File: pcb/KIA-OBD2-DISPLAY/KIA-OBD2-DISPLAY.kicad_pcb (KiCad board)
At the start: 4 copper layers, 132.1 x 19 mm, 58 parts, among them J1 Conn_01x07_Pin, J2 Conn_01x01, J3 Conn_01x01, J4 Conn_01x01, J5 Conn_01x01, J6 Conn_01x01, J7 Conn_01x01, J8 Conn_01x01, J9 Conn_01x01, P1 USB_C_Plug, Q1 BC817, U10 MCP2515-xST, U11 MCP2515-xST, U4 CAP1188-1-CP-TR, U6 TJA1050, U7 TJA1050, U9 ESP32-C6-MINI-1/U, Y1 Crystal_GND24_Small, Y4 Crystal_GND24_Small

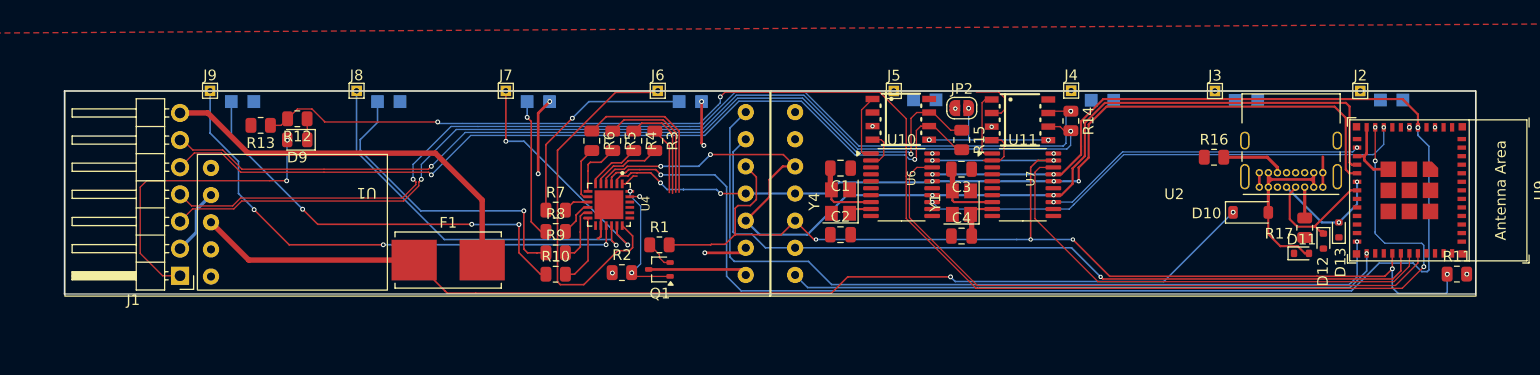
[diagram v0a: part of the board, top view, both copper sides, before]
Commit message: finall pcb
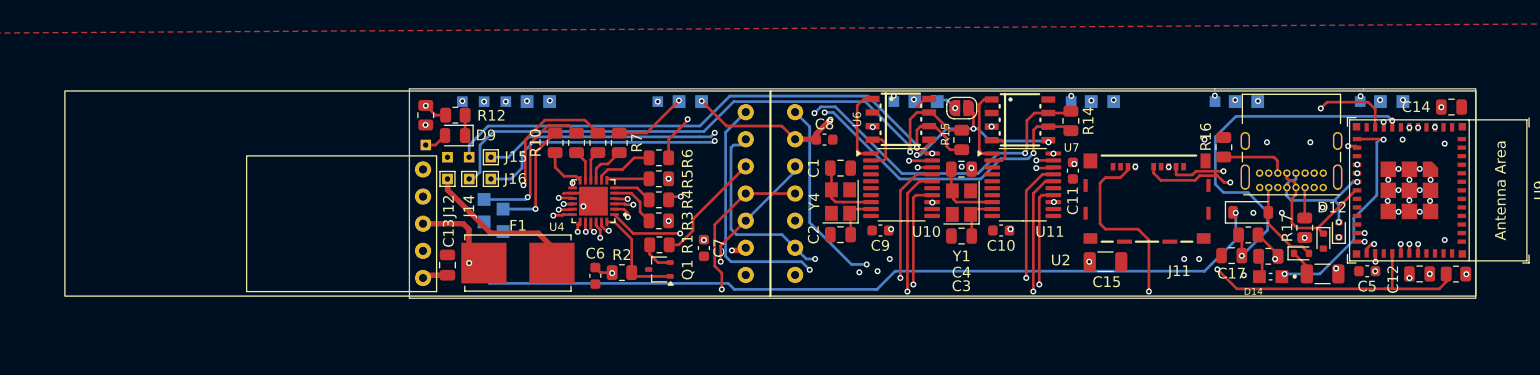
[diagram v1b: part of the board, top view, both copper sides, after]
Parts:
- removed J1: Conn_01x07_Pin, Connector_PinHeader_2.54mm:PinHeader_1x07_P2.54mm_Horizontal
- removed P1: USB_C_Plug, Connector_USB:USB_C_Receptacle_GCT_USB4085
- added C10: 100nF, Capacitor_SMD:C_0603_1608Metric, F.Cu at (181.0, 91.1)
- added C11: 100nF, Capacitor_SMD:C_0603_1608Metric, F.Cu at (187.7, 85.5)
- added C12: 10uF, Capacitor_SMD:C_0805_2012Metric, F.Cu at (220.2, 95.1)
- added C13: 10uF, Capacitor_SMD:C_0805_2012Metric, F.Cu at (129.2, 94.3)
- added C14: 10uF, Capacitor_SMD:C_0805_2012Metric, F.Cu at (223.1, 79.5)
- added C15: 100uF, Capacitor_SMD:C_1206_3216Metric, F.Cu at (190.8, 94.0)
- added C16: 100uF, Capacitor_SMD:C_1206_3216Metric, F.Cu at (211.1, 95.1)
- added C17: 10uF, Capacitor_SMD:C_0805_2012Metric, F.Cu at (202.6, 93.4)
- added C5: 100nF, Capacitor_SMD:C_0603_1608Metric, F.Cu at (215.3, 94.9)
- added C6: 100nF, Capacitor_SMD:C_0603_1608Metric, F.Cu at (143.0, 95.3)
- added C7: 100nF, Capacitor_SMD:C_0603_1608Metric, F.Cu at (153.2, 92.7)
- added C8: 100nF, Capacitor_SMD:C_0603_1608Metric, F.Cu at (164.5, 82.5)
- added C9: 100nF, Capacitor_SMD:C_0603_1608Metric, F.Cu at (169.7, 91.1)
- added D14: LED, LED_0602:LED_QBLP617-IW, F.Cu at (206.2, 95.4)
- added J10: USB_C_Receptacle_USB2.0_16P, Connector_USB:USB_C_Receptacle_GCT_USB4085, F.Cu at (211.1, 87.0)
- added J11: MEM2085-00-115-00-A_REV0.2, MEM2085:GCT_MEM2085-00-115-00-A_REV0.2, F.Cu at (194.6, 88.1)
- added J12: Conn_01x01, TestPoint:TestPoint_THTPad_1.0x1.0mm_Drill0.5mm, F.Cu at (129.2, 86.2)
- added J13: Conn_01x01, TestPoint:TestPoint_THTPad_1.0x1.0mm_Drill0.5mm, B.Cu at (131.2, 84.2)
- added J14: Conn_01x01, TestPoint:TestPoint_THTPad_1.0x1.0mm_Drill0.5mm, F.Cu at (131.2, 86.2)
- added J15: Conn_01x01, TestPoint:TestPoint_THTPad_1.0x1.0mm_Drill0.5mm, F.Cu at (133.2, 84.2)
- added J16: Conn_01x01, TestPoint:TestPoint_THTPad_1.0x1.0mm_Drill0.5mm, F.Cu at (133.2, 86.2)
- added J17: Conn_01x01, TestPoint:TestPoint_THTPad_1.0x1.0mm_Drill0.5mm, B.Cu at (129.2, 84.2)
- added J18: Conn_01x01, TestPoint:TestPoint_THTPad_1.0x1.0mm_Drill0.5mm, B.Cu at (127.1, 83.1)
- added R18: R, Resistor_SMD:R_0805_2012Metric, F.Cu at (206.0, 93.5)
- added R19: R, Resistor_SMD:R_0805_2012Metric, F.Cu at (204.1, 91.5)
- J2, J3, J4, J5, J6, J7, J8, J9: footprint TestPoint:TestPoint_THTPad_1.0x1.0mm_Drill0.5mm -> TestPoint:TestPoint_Pad_1.0x1.0mm; moved to B.Cu
- moved J2 43.7 mm to (170.9, 79.0), turned to 180 degrees
- moved J5 43.7 mm to (214.6, 79.0), turned to 180 degrees
- moved J9 41.9 mm to (148.8, 79.0), turned to 180 degrees
- moved D8 26.8 mm to (134.4, 90.1), turned to 90 degrees
- moved U8 25.8 mm to (128.1, 96.8), turned to 180 degrees
- moved J6 18.3 mm to (130.6, 79.0), turned to 180 degrees
- moved R13 15.5 mm to (127.1, 80.3), turned to -90 degrees
- moved R12 14.8 mm to (129.9, 80.3)
- moved D9 14.8 mm to (129.9, 82.2)
- moved J8 14.0 mm to (134.6, 79.0), turned to 180 degrees
- moved D7 13.6 mm to (132.6, 89.2), turned to 90 degrees
- moved J4 13.5 mm to (201.0, 79.0), turned to 180 degrees
- moved J3 13.5 mm to (187.5, 79.0), turned to 180 degrees
- moved R10 12.3 mm to (139.2, 82.9), turned to -90 degrees
- moved R9 10.5 mm to (141.2, 82.9), turned to -90 degrees
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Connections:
- U9 pad 12: unconnected-(U9-GPIO0/ADC1_CH0/XTAL_32K_P-Pad12) -> Net-(D14-A)
- U9 pad 23: unconnected-(U9-GPIO9-Pad23) -> /CSSDCARD
- U9 pad 30: /CSCAN2 -> /CSCAN
- U9 pad 31: /CSCAN -> /CSCAN2
- U9 pad 8: unconnected-(U9-EN/CHIP_PU-Pad8) -> Net-(U9-EN/CHIP_PU)
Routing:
- net /INTCAP: track 0.00 -> 87.6 mm, vias 1 -> 2
- net Net-(J5-Pin_1): track 0.00 -> 87.3 mm, vias 0 -> 2
- net /CSCAP: track 1.68 -> 77.0 mm, vias 0 -> 2
- net Net-(D1-K): track 6.31 -> 78.3 mm, vias 0 -> 2
- net Net-(J4-Pin_1): track 0.00 -> 68.5 mm, vias 0 -> 2
- net Net-(J3-Pin_1): track 0.00 -> 56.7 mm, vias 0 -> 2
- net /MOSI: track 82.9 -> 138.1 mm, vias 5 -> 6
- net Net-(D2-K): track 9.92 -> 59.1 mm, vias 0 -> 2
- net /INTING: track 141.7 -> 94.8 mm, vias 5 -> 2
- net Net-(J2-Pin_1): track 0.00 -> 37.7 mm, vias 0 -> 2
- net Net-(U9-EN/CHIP_PU): track 0.00 -> 35.8 mm, vias 0 -> 2
- net /MISO: track 154.3 -> 119.5 mm, vias 4 -> 5
- net /CAN LISTEN H: track 97.2 -> 62.9 mm, vias 2 -> 3
- net Net-(J9-Pin_1): track 48.8 -> 15.8 mm, vias 3 -> 2
- net Net-(D3-K): track 12.4 -> 42.6 mm, vias 0 -> 2
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- added copper zone on In2.Cu, net +3.3V
- added copper zone on In1.Cu, net GND
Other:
- board size 132.1 x 19 mm -> 99.8 x 19.6 mm
- rule pad_to_mask_clearance: 0 -> 0.038
- rule solder_mask_min_width: 0.1016 -> 0.1

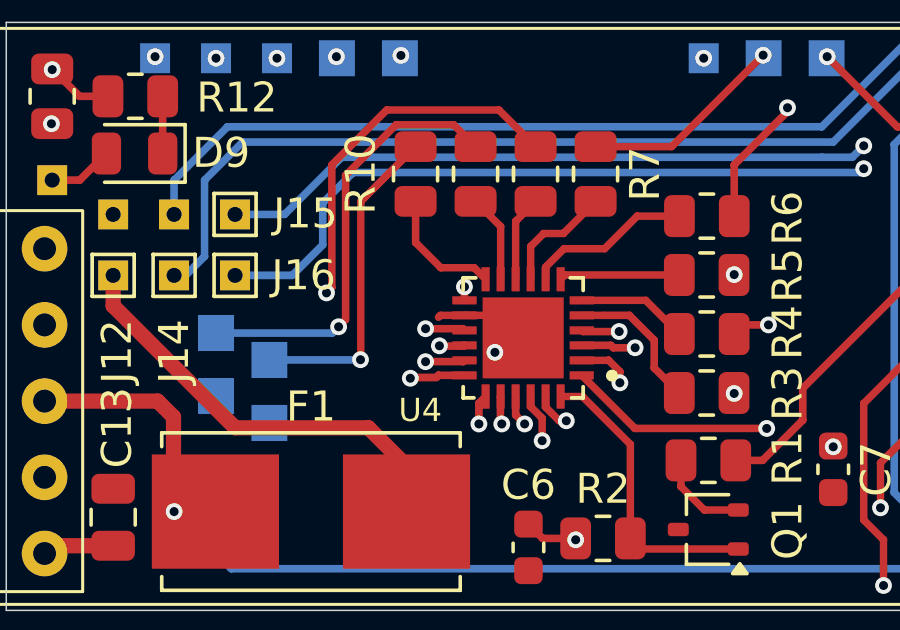
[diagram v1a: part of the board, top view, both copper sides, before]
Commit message: deps and pcb update
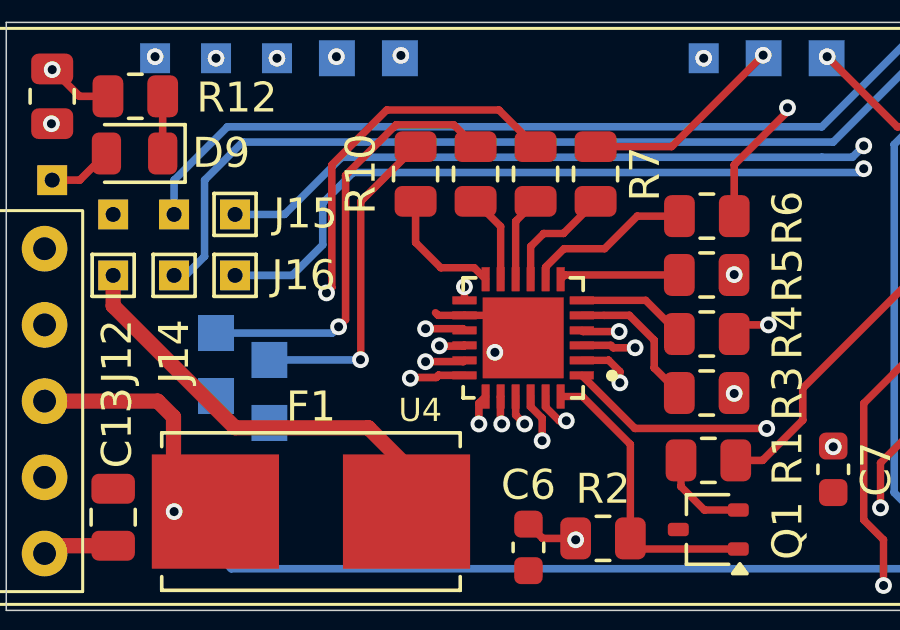
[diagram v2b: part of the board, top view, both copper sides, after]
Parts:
- R10, R18, R3, R4, R5, R6, R7, R8, R9: value R -> 65R
- R11, R19: value R -> 10k
- R12: value R -> 4.7k
- R13: value R -> 1k
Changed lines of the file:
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@@
 			(layer "F.SilkS")
 		)
-		(fp_text user "${REFERENCE}"
-			(at 9.948955 6.206265 180)
-			(unlocked yes)
-			(layer "F.Fab")
-			(effects
-				(font
-					(size 1 1)
-					(thickness 0.15)
-				)
-			)
-		)
 		(pad "1" thru_hole circle
 			(at 1.27 1.27 180)
@@
 			)
 		)
-		(property "Value" "R"
+		(property "Value" "65R"
 			(at 0 1.65 0)
 			(layer "F.Fab")
@@
 			(at 0 4.2 0)
 			(layer "F.Fab")
+			(hide yes)
 			(effects
 				(font
@@
 			)
 		)
-		(property "Value" "R"
+		(property "Value" "65R"
 			(at 0 1.65 90)
 			(layer "F.Fab")
+			(hide yes)
 			(effects
 				(font
@@
 			(at 0 2.45 -90)
 			(layer "F.Fab")
+			(hide yes)
 			(effects
 				(font
@@
 			(at 0 4.2 0)
 			(layer "F.Fab")
+			(hide yes)
 			(effects
 				(font
@@
 		)
 		(property "Value" "22pF"
-			(at 0 1.68 180)
+			(at 2.754282 0.12994 -90)
 			(layer "F.Fab")
 			(effects
@@
 			)
 		)
-		(property "Value" "R"
+		(property "Value" "65R"
 			(at 0 1.65 0)
 			(layer "F.Fab")
+			(hide yes)
 			(effects
 				(font
@@
 		)
 		(property "Value" "100nF"
-			(at 0 1.43 0)
+			(at -0.902 -1.778 0)
 			(layer "F.Fab")
 			(effects
@@
 			)
 		)
-		(property "Value" "R"
+		(property "Value" "65R"
 			(at 0 1.65 0)
 			(layer "F.Fab")
+			(hide yes)
 			(effects
 				(font
@@
 			)
 		)
-		(property "Value" "R"
+		(property "Value" "65R"
 			(at 0 1.65 90)
 			(layer "F.Fab")
@@
 		)
 		(property "Value" "TJA1050"
-			(at 6.5 0.5 90)
+			(at -4.119 -0.003 180)
 			(layer "F.Fab")
 			(effects
@@
 		)
 		(property "Value" "100nF"
-			(at 0 1.43 0)
+			(at -0.114 -1.778 0)
 			(layer "F.Fab")
 			(effects
@@
 			(at 7.95 1.95 180)
 			(layer "F.Fab")
+			(hide yes)
 			(effects
 				(font
@@
 		)
 		(property "Value" "5.1k"
-			(at 0 1.65 90)
+			(at -1.858128 1.804804 90)
 			(layer "F.Fab")
 			(effects
@@
 			(at 0 1.85 0)
 			(layer "F.Fab")
-			(hide yes)
 			(effects
 				(font
@@
 			)
 		)
-		(property "Value" "R"
+		(property "Value" "10k"
 			(at 0 1.65 0)
 			(layer "F.Fab")
@@
 		)
 		(property "Value" "SD05_SOD323"
-			(at 0 1.4 0)
+			(at -3.995 5.86 0)
 			(layer "F.Fab")
-			(hide yes)
 			(effects
 				(font
@@
 		)
 		(fp_text user "${REFERENCE}"
-			(at 0 -1.3 0)
+			(at -1.963 -1.633 0)
 			(layer "F.Fab")
 			(effects
@@
 		)
 		(property "Value" "100nF"
-			(at 0 1.43 90)
+			(at 3.823 0 90)
 			(layer "F.Fab")
 			(effects
@@
 		)
 		(property "Value" "100nF"
-			(at 0 1.43 0)
+			(at -1.257 -1.778 0)
 			(layer "F.Fab")
 			(effects
@@
 			)
 		)
-		(property "Value" "R"
-			(at 0 1.65 0)
+		(property "Value" "65R"
+			(at 0 3.81 0)
 			(layer "F.Fab")
 			(effects
@@
 			)
 		)
-		(property "Value" "R"
+		(property "Value" "65R"
 			(at 0 1.65 0)
 			(layer "F.Fab")
+			(hide yes)
 			(effects
 				(font
@@
 		)
 		(property "Value" "10uF"
-			(at 0 1.68 0)
+			(at 1.649364 -2.224239 0)
 			(layer "F.Fab")
 			(effects
@@
 		)
 		(property "Value" "100nF"
-			(at 0 1.43 0)
+			(at -0.876 -1.778 0)
 			(layer "F.Fab")
 			(effects
@@
 		)
 		(property "Value" "22pF"
-			(at 0 1.68 180)
+			(at -0.018646 -1.678598 0)
 			(layer "F.Fab")
 			(effects
@@
 		)
 		(property "Value" "TJA1050"
-			(at 6.5 0.5 90)
+			(at -4.069 0.020975 180)
 			(layer "F.Fab")
 			(effects
@@
 		)
 		(property "Value" "100uF"
-			(at 0 1.85 0)
+			(at 0 -2.032 0)
 			(layer "F.Fab")
 			(effects
@@
 		)
 		(fp_text user "${REFERENCE}"
-			(at 0 -1.3 -90)
+			(at 0.068 2.665 0)
 			(layer "F.Fab")
 			(effects
@@
 		)
 		(property "Value" "5.1k"
-			(at 0 1.65 -90)
+			(at 1.646 -1.755 -90)
 			(layer "F.Fab")
-			(hide yes)
 			(effects
 				(font
@@
 		)
 		(property "Value" "10uF"
-			(at 0 1.68 0)
+			(at -0.315 -2.159 0)
 			(layer "F.Fab")
 			(effects
@@
 		)
 		(fp_text user "${REFERENCE}"
-			(at 0 -1.3 90)
+			(at -2.769 0.076 -90)
 			(layer "F.Fab")
 			(effects
@@
 		)
 		(property "Value" "10uF"
-			(at 0 1.68 0)
+			(at 0 -1.905 0)
 			(layer "F.Fab")
 			(effects
@@
 		)
 		(property "Value" "BC817"
-			(at -0.05 2.05 180)
+			(at -0.227313 -2.57776 180)
 			(layer "F.Fab")
 			(effects
@@
 			)
 		)
-		(property "Value" "R"
+		(property "Value" "4.7k"
 			(at 0 1.65 180)
 			(layer "F.Fab")
@@
 			)
 		)
-		(property "Value" "R"
+		(property "Value" "1k"
 			(at 0 1.65 90)
 			(layer "F.Fab")
@@
 		)
 		(property "Value" "120R"
-			(at 0 1.65 90)
+			(at 0.224859 -1.972484 90)
 			(layer "F.Fab")
 			(effects
@@
 			(at 12.85 -5.315 0)
 			(layer "F.Fab")
+			(hide yes)
 			(effects
 				(font
@@
 			)
 		)
-		(property "Value" "R"
+		(property "Value" "65R"
 			(at 0 1.65 90)
 			(layer "F.Fab")
+			(hide yes)
 			(effects
 				(font
@@
 			(at 0 2.45 -90)
 			(layer "F.Fab")
+			(hide yes)
 			(effects
 				(font
@@
 			(at 0 1.9 0)
 			(layer "F.Fab")
+			(hide yes)
 			(effects
 				(font
@@
 		)
 		(property "Value" "100nF"
-			(at 0 1.43 90)
+			(at 2.68 -0.508 180)
 			(layer "F.Fab")
 			(effects
@@
 		)
 		(property "Value" "100nF"
-			(at 0 1.43 90)
+			(at 3.1242 0.635 180)
 			(layer "F.Fab")
 			(effects
@@
 			)
 		)
-		(property "Value" "R"
-			(at 0 1.65 0)
+		(property "Value" "10k"
+			(at 3.106765 0.082492 0)
 			(layer "F.Fab")
 			(effects
@@
 			)
 		)
-		(property "Value" "R"
+		(property "Value" "65R"
 			(at 0 1.65 90)
 			(layer "F.Fab")
@@
 		)
 		(property "Value" "120R"
-			(at 0 1.65 90)
+			(at -5.749411 -0.122566 0)
 			(layer "F.Fab")
 			(effects
@@
 			(at 0 -1.55 0)
 			(layer "B.Fab")
+			(hide yes)
 			(effects
 				(font
@@
 			(at 0 -1.55 0)
 			(layer "B.Fab")
+			(hide yes)
 			(effects
 				(font
@@
 			(at 0 -1.55 0)
 			(layer "B.Fab")
+			(hide yes)
 			(effects
 				(font
@@
 			(at 0 -1.55 0)
 			(layer "B.Fab")
+			(hide yes)
 			(effects
 				(font
@@
 	)
 	(segment
-		(start 140.0698 87.565)
-		(end 140.0048 87.63)
+		(start 139.9906 87.565)
+		(end 139.9032 87.4776)
 		(width 0.25)
 		(layer "F.Cu")
@@
 	(segment
 		(start 140.8715 87.565)
-		(end 140.0698 87.565)
+		(end 139.9906 87.565)
 		(width 0.25)
 		(layer "F.Cu")
